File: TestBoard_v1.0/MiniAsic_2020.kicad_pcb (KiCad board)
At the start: 2 copper layers, 70 x 40 mm, 23 parts, among them J1 Screw_Terminal_01x04, J2 Conn_Coaxial, J3 Conn_Coaxial

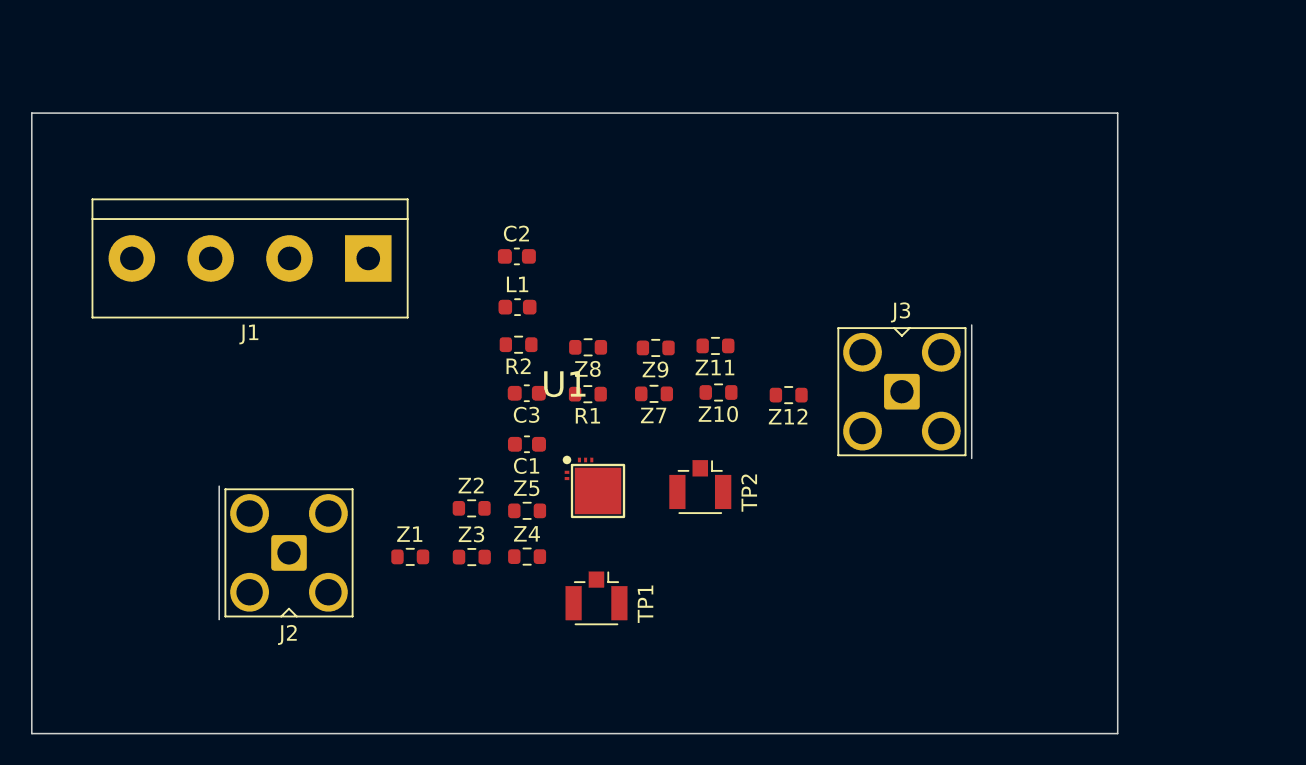
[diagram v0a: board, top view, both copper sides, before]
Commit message: Initial routing
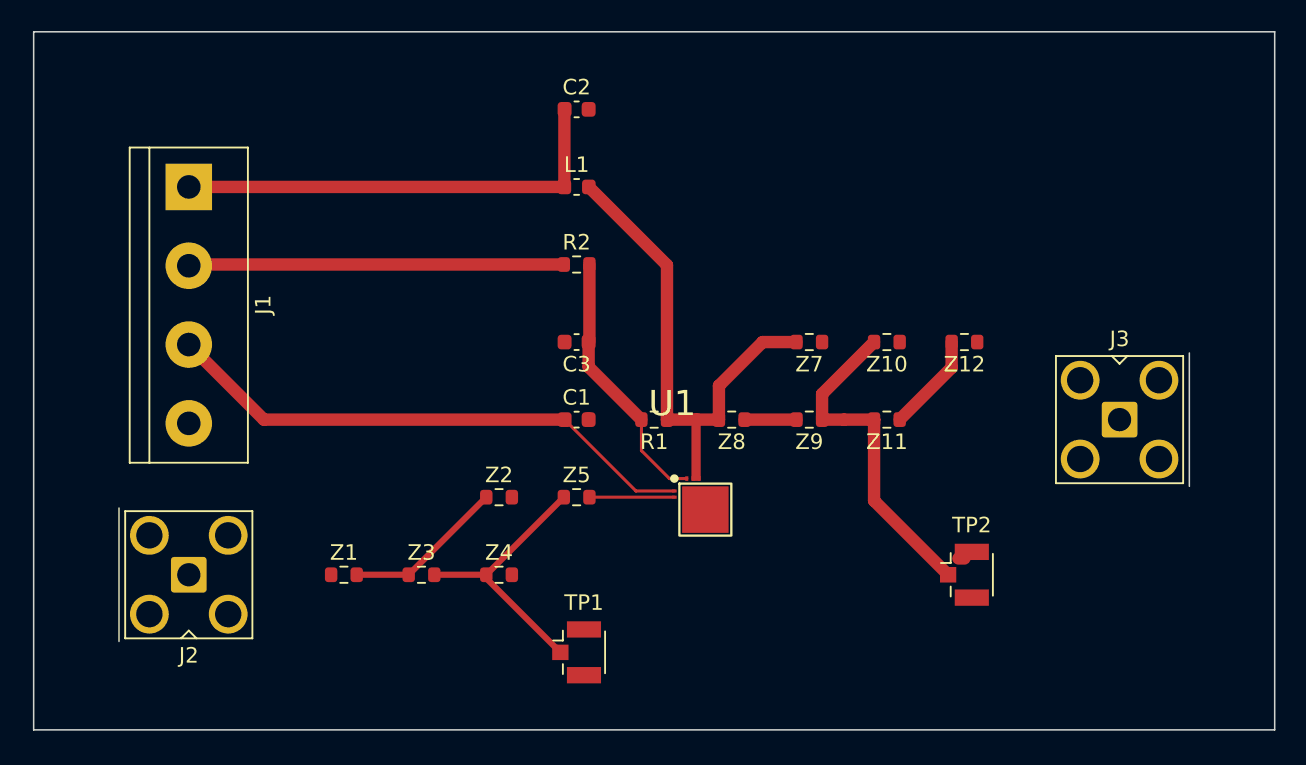
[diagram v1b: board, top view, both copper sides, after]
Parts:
- moved TP2 18.0 mm to (205.0, 130.0), turned to 0 degrees
- moved J3 14.1 mm to (215.0, 120.0)
- moved J1 12.5 mm to (155.0, 105.0), turned to -90 degrees
- moved Z11 12.0 mm to (200.0, 120.0)
- moved Z12 11.8 mm to (205.0, 115.0)
- moved Z10 11.3 mm to (200.0, 115.0)
- moved Z9 10.9 mm to (195.0, 120.0)
- moved Z7 10.6 mm to (195.0, 115.0)
- moved Z8 10.4 mm to (190.0, 120.0)
- moved C2 10.2 mm to (180.0, 100.0)
- moved L1 8.64 mm to (180.0, 105.0)
- moved U1 7.02 mm to (186.8, 124.3)
- moved J2 6.61 mm to (155.0, 130.0)
- moved R2 6.38 mm to (180.0, 110.0)
- moved C3 4.60 mm to (180.0, 115.0)
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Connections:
- TP1 pad 1: Net-(#PWR030-GND) -> /TP1
- TP1 pad 2: /TP1 -> Net-(TP1-GND)
- TP2 pad 1: Net-(#PWR031-GND) -> /TP2
- TP2 pad 2: /TP2 -> Net-(TP2-GND)
- Z10 pad 2: Net-(Z10-Pad2) -> /TP2
- Z11 pad 1: /TP2 -> Net-(T2-Pad1)
- Z11 pad 2: Net-(Z10-Pad2) -> /TP2
- Z12 pad 2: /TP2 -> Net-(T2-Pad1)
- Z9 pad 1: Net-(Z10-Pad2) -> /TP2
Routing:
- net +1V8: track 0.00 -> 35.2 mm
- net +3.3V: track 0.00 -> 29.2 mm
- net /OUT: track 0.00 -> 28.8 mm
- net /VG: track 0.00 -> 24.3 mm
- net /TP2: track 0.00 -> 21.7 mm
- net /TP1: track 0.00 -> 17.4 mm
- net /VG_GATED: track 0.00 -> 17.2 mm
- net Net-(Z1-Pad2): track 0.00 -> 10.4 mm
- net Net-(T2-Pad1): track 0.00 -> 6.39 mm
- net /IN: track 0.00 -> 5.48 mm
- net Net-(Z8-Pad1): track 0.00 -> 3.35 mm
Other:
- board size 70 x 40 mm -> 80 x 45 mm
